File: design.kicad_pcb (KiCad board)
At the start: 2 copper layers, 25 x 22.9 mm, 1 part, among them J1 USB4130-GF-C

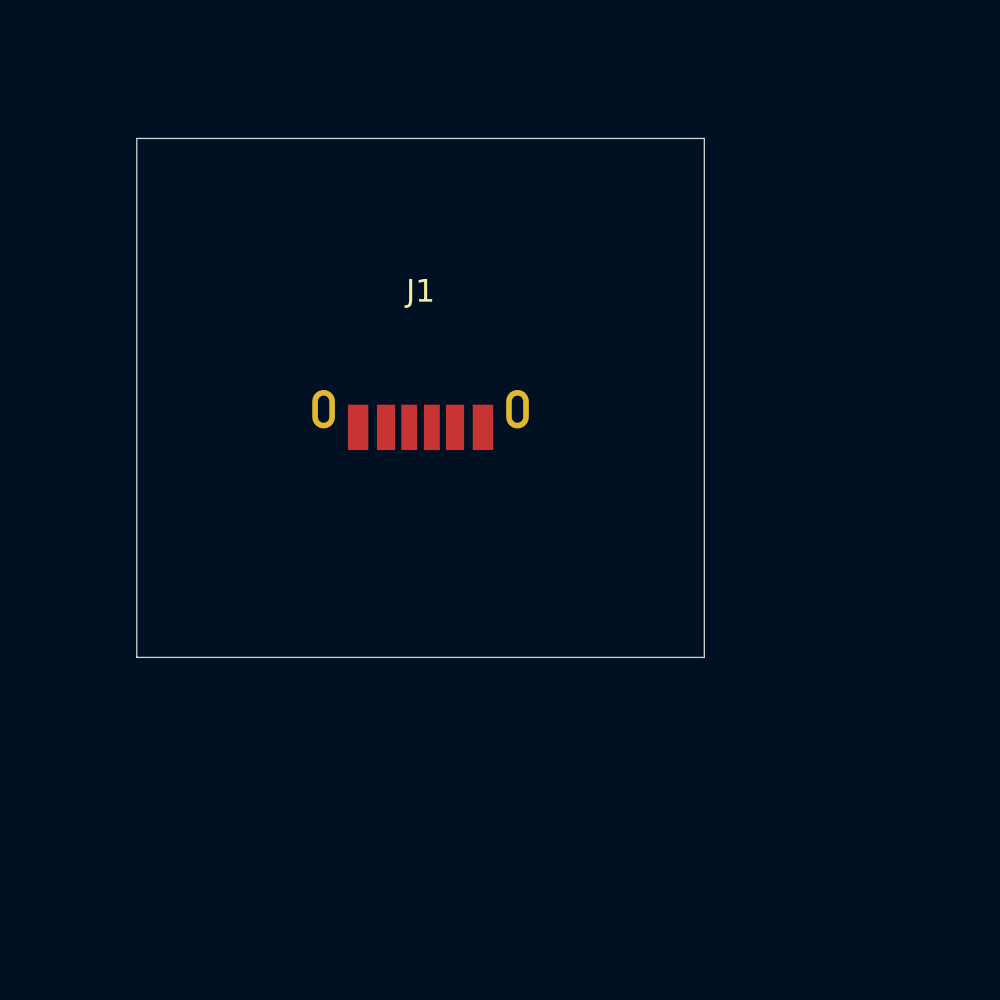
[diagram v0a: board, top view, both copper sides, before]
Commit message: PCB&SCH update
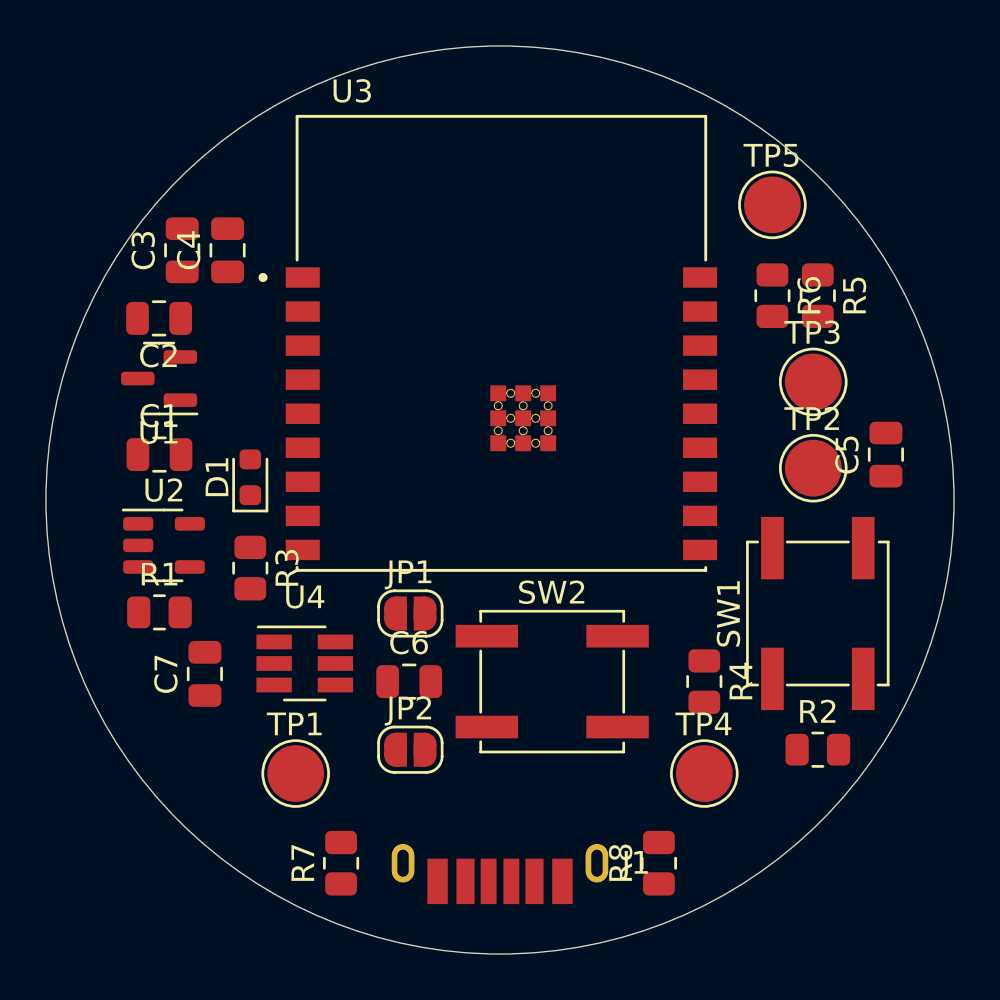
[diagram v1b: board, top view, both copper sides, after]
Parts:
- added C1: 1uF, Capacitor_SMD:C_0805_2012Metric, F.Cu at (135.0, 98.0)
- added C2: 1uF, Capacitor_SMD:C_0805_2012Metric, F.Cu at (135.0, 92.0)
- added C3: 10uF, Capacitor_SMD:C_0805_2012Metric, F.Cu at (136.0, 89.0)
- added C4: 0.1uF, Capacitor_SMD:C_0805_2012Metric, F.Cu at (138.0, 89.0)
- added C5: 1uF, Capacitor_SMD:C_0805_2012Metric, F.Cu at (167.0, 98.0)
- added C6: 100nF, Capacitor_SMD:C_0805_2012Metric, F.Cu at (146.0, 108.0)
- added C7: 0-50pF, Capacitor_SMD:C_0805_2012Metric, F.Cu at (137.0, 107.7)
- added D1: LED, LED_SMD:LED_0603_1608Metric, F.Cu at (139.0, 99.0)
- added JP1: TOG, Jumper:SolderJumper-2_P1.3mm_Open_RoundedPad1.0x1.5mm, F.Cu at (146.1, 105.0)
- added JP2: AHLB, Jumper:SolderJumper-2_P1.3mm_Open_RoundedPad1.0x1.5mm, F.Cu at (146.1, 111.0)
- added R1: 10K, Resistor_SMD:R_0805_2012Metric, F.Cu at (135.0, 105.0)
- added R2: 10K, Resistor_SMD:R_0805_2012Metric, F.Cu at (164.0, 111.0)
- added R3: 470, Resistor_SMD:R_0805_2012Metric, F.Cu at (139.0, 103.0)
- added R4: 10K, Resistor_SMD:R_0805_2012Metric, F.Cu at (159.0, 108.0)
- added R5: 10K, Resistor_SMD:R_0805_2012Metric, F.Cu at (164.0, 91.0)
- added R6: 10K, Resistor_SMD:R_0805_2012Metric, F.Cu at (162.0, 91.0)
- added R7: 5.1k, Resistor_SMD:R_0805_2012Metric, F.Cu at (143.0, 116.0)
- added R8: 5.1k, Resistor_SMD:R_0805_2012Metric, F.Cu at (157.0, 116.0)
- added SW1: EN, Button_Switch_SMD:SW_SPST_EVPBF, F.Cu at (164.0, 105.0)
- added SW2: IO9, Button_Switch_SMD:SW_SPST_EVPBF, F.Cu at (152.3, 108.0)
- added TP1: GND, TestPoint:TestPoint_Pad_D2.5mm, F.Cu at (141.0, 112.0)
- added TP2: D-, TestPoint:TestPoint_Pad_D2.5mm, F.Cu at (163.8, 98.6)
- added TP3: D+, TestPoint:TestPoint_Pad_D2.5mm, F.Cu at (163.8, 94.8)
- added TP4: +BATT, TestPoint:TestPoint_Pad_D2.5mm, F.Cu at (159.0, 112.0)
- added TP5: +3.3V, TestPoint:TestPoint_Pad_D2.5mm, F.Cu at (162.0, 87.0)
- added U1: MCP1700-3302E_SOT23, Package_TO_SOT_SMD:SOT-23, F.Cu at (135.0, 94.7)
- added U2: TCK108AF,LF, Package_TO_SOT_SMD:SOT-23-5, F.Cu at (135.2, 102.0)
- added U3: ESP32-C3-WROOM-02-N4, MCU_Espressif_custom:MODULE_ESP32-C3-WROOM-02-H4, F.Cu at (150.1, 93.1)
- added U4: TTP223, Package_TO_SOT_SMD:SOT-23-6_Handsoldering, F.Cu at (141.4, 107.2)
- moved J1 20.3 mm to (150.0, 116.0)
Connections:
- net Net-(J1-PadA12) renamed GND
- net Net-(J1-PadA9) renamed +BATT
- J1 pad A5: unconnected-(J1-PadA5) -> Net-(J1-PadA5)
- J1 pad B5: unconnected-(J1-PadB5) -> Net-(J1-PadB5)
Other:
- board size 25 x 22.9 mm -> 40 x 40 mm
